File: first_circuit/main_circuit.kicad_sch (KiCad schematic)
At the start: 3 parts

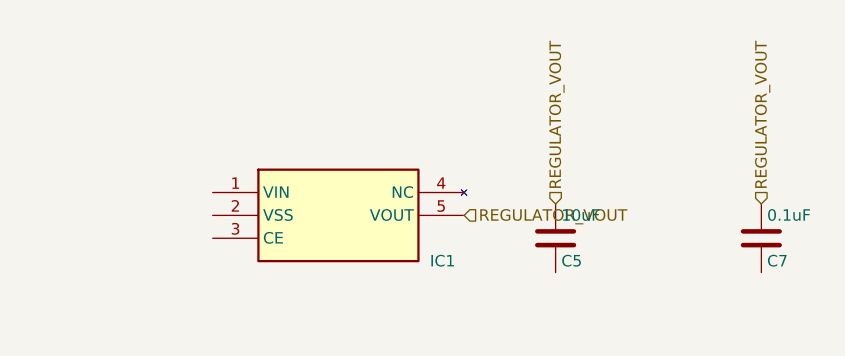
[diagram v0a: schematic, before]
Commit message: start again
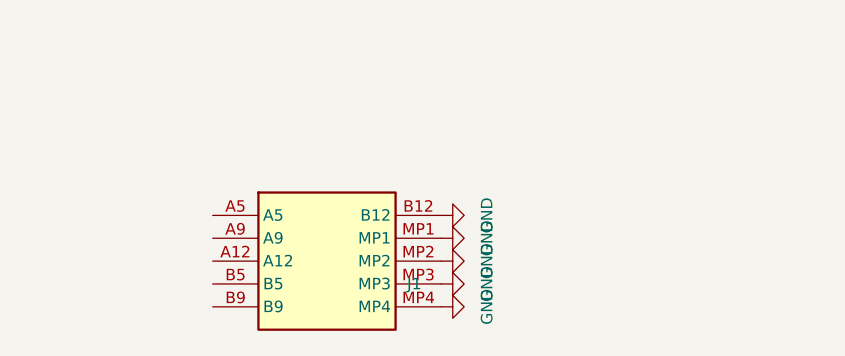
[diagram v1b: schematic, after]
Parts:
- removed C5: 10uF, Capacitor_SMD:C_0201_0603Metric, symbol Device:C
- removed C7: 0.1uF, Capacitor_SMD:C_0201_0603Metric, symbol Device:C
- removed IC1: (no value), SamacSys_Parts:SOT95P280X130-5N, symbol SamacSys_Parts:XC6220B331MR-G
- added J1: (no value), SamacSys_Parts:USB4135GFA, symbol SamacSys_Parts:USB4135-GF-A
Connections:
- new net GND: J1.B12, J1.MP1, J1.MP2, J1.MP3, J1.MP4

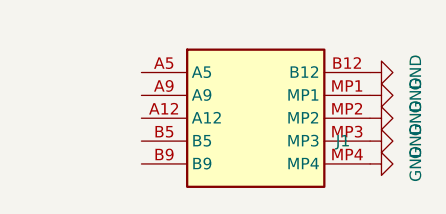
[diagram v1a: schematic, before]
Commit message: rc_delay
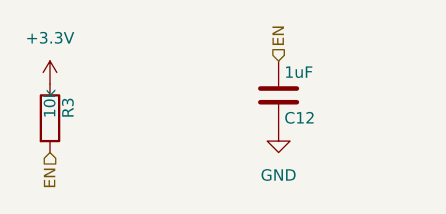
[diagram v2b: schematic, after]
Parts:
- removed J1: (no value), SamacSys_Parts:USB4135GFA, symbol SamacSys_Parts:USB4135-GF-A
- added C12: 1uF, Capacitor_SMD:C_0603_1608Metric, symbol Device:C
- added R3: 10k, Resistor_SMD:R_0603_1608Metric, symbol Device:R
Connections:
- net GND: now also C12.2
- new net +3.3V: R3.1
- new net EN: C12.1, R3.2
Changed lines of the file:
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@@
 	)
 	(symbol
-		(lib_id "SamacSys_Parts:USB4135-GF-A")
-		(at 40.64 30.48 0)
-		(unit 1)
-		(exclude_from_sim no)
-		(in_bom yes)
-		(on_board yes)
-		(dnp no)
-		(fields_autoplaced no)
-		(property "Reference" "J1"
-			(at 62.23 38.1 0.0000)
-			(effects
-				(font
-					(size 1.27 1.27)
-				)
-				(justify left)
-			)
-		)
-		(property "Footprint" "SamacSys_Parts:USB4135GFA"
-			(at 62.23 -64.44 0.0000)
-			(effects
-				(font
-					(size 1.27 1.27)
-				)
-				(hide yes)
-			)
-		)
-		(property "hierarchy_path" "/74824406-cd07-43be-b55f-f7d501532b0e"
-			(at 43.18 35.5599 0)
+		(lib_id "Device:R")
+		(at 30.48 35.56 0)
+		(unit 1)
+		(exclude_from_sim no)
+		(in_bom yes)
+		(on_board yes)
+		(dnp no)
+		(fields_autoplaced no)
+		(property "Reference" "R3"
+			(at 32.512 35.56 90)
+			(effects
+				(font
+					(size 1.27 1.27)
+				)
+				(justify left)
+			)
+		)
+		(property "Value" "10k"
+			(at 30.48 35.56 90)
+			(effects
+				(font
+					(size 1.27 1.27)
+				)
+				(justify left)
+			)
+		)
+		(property "Footprint" "Resistor_SMD:R_0603_1608Metric"
+			(at 28.702 35.56 90)
+			(effects
+				(font
+					(size 1.27 1.27)
+				)
+				(hide yes)
+			)
+		)
+		(property "hierarchy_path" "/18790e42-201e-4808-bfa1-f33409c8c696"
+			(at 33.02 40.6399 0)
 			(effects
 				(font
@@
 		)
 		(property "project_name" "main_circuit"
-			(at 43.18 35.5599 0)
-			(effects
-				(font
-					(size 1.27 1.27)
-				)
-				(hide yes)
-			)
-		)
-		(property "root_uuid" "74824406-cd07-43be-b55f-f7d501532b0e"
-			(at 43.18 35.5599 0)
-			(effects
-				(font
-					(size 1.27 1.27)
-				)
-				(hide yes)
-			)
-		)
-		(pin "A5"
-		)
-		(pin "A9"
-		)
-		(pin "A12"
-		)
-		(pin "B5"
-		)
-		(pin "B9"
-		)
-		(pin "B12"
-		)
-		(pin "MP1"
-		)
-		(pin "MP2"
-		)
-		(pin "MP3"
-		)
-		(pin "MP4"
-		)
-		(instances
-			(project ""
-				(path "/74824406-cd07-43be-b55f-f7d501532b0e"
-					(reference "J1")
-					(unit 1)
-				)
-			)
-		)
-	)
-	(symbol
-		(lib_id "power:GND")
-		(at 66.04 30.48 90)
+			(at 33.02 40.6399 0)
+			(effects
+				(font
+					(size 1.27 1.27)
+				)
+				(hide yes)
+			)
+		)
+		(property "root_uuid" "18790e42-201e-4808-bfa1-f33409c8c696"
+			(at 33.02 40.6399 0)
+			(effects
+				(font
+					(size 1.27 1.27)
+				)
+				(hide yes)
+			)
+		)
+		(pin "1"
+		)
+		(pin "2"
+		)
+		(instances
+			(project ""
+				(path "/18790e42-201e-4808-bfa1-f33409c8c696"
+					(reference "R3")
+					(unit 1)
+				)
+			)
+		)
+	)
+	(symbol
+		(lib_id "Device:C")
+		(at 55.88 33.02 0)
+		(unit 1)
+		(exclude_from_sim no)
+		(in_bom yes)
+		(on_board yes)
+		(dnp no)
+		(fields_autoplaced no)
+		(property "Reference" "C12"
+			(at 56.515 35.56 0.0000)
+			(effects
+				(font
+					(size 1.27 1.27)
+				)
+				(justify left)
+			)
+		)
+		(property "Value" "1uF"
+			(at 56.515 30.48 0.0000)
+			(effects
+				(font
+					(size 1.27 1.27)
+				)
+				(justify left)
+			)
+		)
+		(property "Footprint" "Capacitor_SMD:C_0603_1608Metric"
+			(at 56.8452 29.21 0.0000)
+			(effects
+				(font
+					(size 1.27 1.27)
+				)
+				(hide yes)
+			)
+		)
+		(property "hierarchy_path" "/18790e42-201e-4808-bfa1-f33409c8c696"
+			(at 58.42 38.0999 0)
+			(effects
+				(font
+					(size 1.27 1.27)
+				)
+				(hide yes)
+			)
+		)
+		(property "project_name" "main_circuit"
+			(at 58.42 38.0999 0)
+			(effects
+				(font
+					(size 1.27 1.27)
+				)
+				(hide yes)
+			)
+		)
+		(property "root_uuid" "18790e42-201e-4808-bfa1-f33409c8c696"
+			(at 58.42 38.0999 0)
+			(effects
+				(font
+					(size 1.27 1.27)
+				)
+				(hide yes)
+			)
+		)
+		(pin "1"
+		)
+		(pin "2"
+		)
+		(instances
+			(project ""
+				(path "/18790e42-201e-4808-bfa1-f33409c8c696"
+					(reference "C12")
+					(unit 1)
+				)
+			)
+		)
+	)
+	(symbol
+		(lib_id "power:+3V3")
+		(at 30.48 31.75 0)
 		(unit 1)
 		(exclude_from_sim no)
@@
 		(fields_autoplaced no)
 		(property "Reference" "#PWR001"
-			(at 72.39 30.48 90)
-			(effects
-				(font
-					(size 1.27 1.27)
-				)
-				(justify left)
-				(hide yes)
-			)
-		)
-		(property "Value" "GND"
-			(at 71.11999999999999 30.48 0)
+			(at 30.48 27.94 0.0000)
+			(effects
+				(font
+					(size 1.27 1.27)
+				)
+				(justify left)
+				(hide yes)
+			)
+		)
+		(property "Value" "+3.3V"
+			(at 30.48 26.67 0)
 			(effects
 				(font
@@
 		)
 		(property "Footprint" ""
-			(at 66.04 30.48 0.0000)
+			(at 30.48 31.75 0.0000)
 			(effects
 				(font
@@
 	(symbol
 		(lib_id "power:GND")
-		(at 66.04 33.02 90)
+		(at 55.88 36.83 0)
 		(unit 1)
 		(exclude_from_sim no)
@@
 		(fields_autoplaced no)
 		(property "Reference" "#PWR002"
-			(at 72.39 33.02 90)
+			(at 55.88 30.48 0.0000)
 			(effects
 				(font
@@
 		)
 		(property "Value" "GND"
-			(at 71.11999999999999 33.02 0)
+			(at 55.88 41.910000000000004 0)
 			(effects
 				(font
@@
 		)
 		(property "Footprint" ""
-			(at 66.04 33.02 0.0000)
+			(at 55.88 36.83 0.0000)
 			(effects
 				(font
@@
 		)
 	)
-	(symbol
-		(lib_id "power:GND")
-		(at 66.04 35.56 90)
-		(unit 1)
-		(exclude_from_sim no)
-		(in_bom yes)
-		(on_board yes)
-		(dnp no)
-		(fields_autoplaced no)
-		(property "Reference" "#PWR003"
-			(at 72.39 35.56 90)
-			(effects
-				(font
-					(size 1.27 1.27)
-				)
-				(justify left)
-				(hide yes)
-			)
-		)
-		(property "Value" "GND"
-			(at 71.11999999999999 35.56 0)
-			(effects
-				(font
-					(size 1.27 1.27)
-				)
-			)
-		)
-		(property "Footprint" ""
-			(at 66.04 35.56 0.0000)
-			(effects
-				(font
-					(size 1.27 1.27)
-				)
-				(hide yes)
-			)
-		)
-		(pin "1"
-		)
-		(instances
-			(project ""
-				(path "/"
-					(reference "#PWR003")
-					(unit 1)
-				)
-			)
-		)
-	)
-	(symbol
-		(lib_id "power:GND")
-		(at 66.04 38.1 90)
-		(unit 1)
-		(exclude_from_sim no)
-		(in_bom yes)
-		(on_board yes)
-		(dnp no)
-		(fields_autoplaced no)
-		(property "Reference" "#PWR004"
-			(at 72.39 38.1 90)
-			(effects
-				(font
-					(size 1.27 1.27)
-				)
-				(justify left)
-				(hide yes)
-			)
-		)
-		(property "Value" "GND"
-			(at 71.11999999999999 38.1 0)
-			(effects
-				(font
-					(size 1.27 1.27)
-				)
-			)
-		)
-		(property "Footprint" ""
-			(at 66.04 38.1 0.0000)
-			(effects
-				(font
-					(size 1.27 1.27)
-				)
-				(hide yes)
-			)
-		)
-		(pin "1"
-		)
-		(instances
-			(project ""
-				(path "/"
-					(reference "#PWR004")
-					(unit 1)
-				)
-			)
-		)
-	)
-	(symbol
-		(lib_id "power:GND")
-		(at 66.04 40.64 90)
-		(unit 1)
-		(exclude_from_sim no)
-		(in_bom yes)
-		(on_board yes)
-		(dnp no)
-		(fields_autoplaced no)
-		(property "Reference" "#PWR005"
-			(at 72.39 40.64 90)
-			(effects
-				(font
-					(size 1.27 1.27)
-				)
-				(justify left)
-				(hide yes)
-			)
-		)
-		(property "Value" "GND"
-			(at 71.11999999999999 40.64 0)
-			(effects
-				(font
-					(size 1.27 1.27)
-				)
-			)
-		)
-		(property "Footprint" ""
-			(at 66.04 40.64 0.0000)
-			(effects
-				(font
-					(size 1.27 1.27)
-				)
-				(hide yes)
-			)
-		)
-		(pin "1"
-		)
-		(instances
-			(project ""
-				(path "/"
-					(reference "#PWR005")
-					(unit 1)
-				)
-			)
-		)
-	)
+	(hierarchical_label "EN"
+		(shape input)
+		(at 30.48 39.37 270)
+		(effects
+			(font
+				(size 1.27 1.27)
+			)
+			(justify right)
+		)
+	)
+	(hierarchical_label "EN"
+		(shape input)
+		(at 55.88 29.21 90)
+		(effects
+			(font
+				(size 1.27 1.27)
+			)
+			(justify left)
+		)
+	)

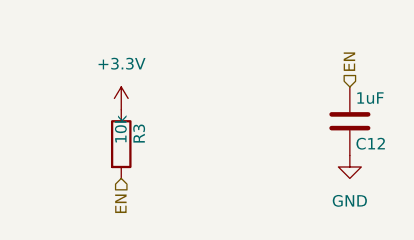
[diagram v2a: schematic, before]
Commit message: uart
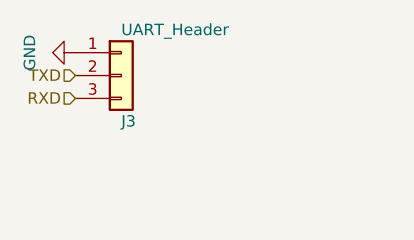
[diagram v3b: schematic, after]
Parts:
- removed C12: 1uF, Capacitor_SMD:C_0603_1608Metric, symbol Device:C
- removed R3: 10k, Resistor_SMD:R_0603_1608Metric, symbol Device:R
- added J3: UART_Header, Connector_PinHeader_2.54mm:PinHeader_1x03_P2.54mm_Vertical, symbol Connector_Generic:Conn_01x03
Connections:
- net GND: now also J3.1 (Pin_1)
- new net RXD: J3.3 (Pin_3)
- new net TXD: J3.2 (Pin_2)
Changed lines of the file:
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@@
 	)
 	(symbol
-		(lib_id "Device:R")
-		(at 30.48 35.56 0)
+		(lib_id "Connector_Generic:Conn_01x03")
+		(at 30.48 27.94 0)
 		(unit 1)
 		(exclude_from_sim no)
@@
 		(dnp no)
 		(fields_autoplaced no)
-		(property "Reference" "R3"
-			(at 32.512 35.56 90)
+		(property "Reference" "J3"
+			(at 30.48 33.02 0.0000)
 			(effects
 				(font
@@
 			)
 		)
-		(property "Value" "10k"
-			(at 30.48 35.56 90)
+		(property "Value" "UART_Header"
+			(at 30.48 22.86 0.0000)
 			(effects
 				(font
@@
 			)
 		)
-		(property "Footprint" "Resistor_SMD:R_0603_1608Metric"
-			(at 28.702 35.56 90)
+		(property "Footprint" "Connector_PinHeader_2.54mm:PinHeader_1x03_P2.54mm_Vertical"
+			(at 30.48 27.94 0.0000)
 			(effects
 				(font
@@
 			)
 		)
-		(property "hierarchy_path" "/18790e42-201e-4808-bfa1-f33409c8c696"
-			(at 33.02 40.6399 0)
+		(property "hierarchy_path" "/d6d32006-2e24-439e-8123-b988d5d2a167"
+			(at 33.02 33.0199 0)
 			(effects
 				(font
@@
 		)
 		(property "project_name" "main_circuit"
-			(at 33.02 40.6399 0)
+			(at 33.02 33.0199 0)
 			(effects
 				(font
@@
 			)
 		)
-		(property "root_uuid" "18790e42-201e-4808-bfa1-f33409c8c696"
-			(at 33.02 40.6399 0)
+		(property "root_uuid" "d6d32006-2e24-439e-8123-b988d5d2a167"
+			(at 33.02 33.0199 0)
 			(effects
 				(font
@@
 		(pin "2"
 		)
+		(pin "3"
+		)
 		(instances
 			(project ""
-				(path "/18790e42-201e-4808-bfa1-f33409c8c696"
-					(reference "R3")
+				(path "/d6d32006-2e24-439e-8123-b988d5d2a167"
+					(reference "J3")
 					(unit 1)
 				)
@@
 	)
 	(symbol
-		(lib_id "Device:C")
-		(at 55.88 33.02 0)
-		(unit 1)
-		(exclude_from_sim no)
-		(in_bom yes)
-		(on_board yes)
-		(dnp no)
-		(fields_autoplaced no)
-		(property "Reference" "C12"
-			(at 56.515 35.56 0.0000)
-			(effects
-				(font
-					(size 1.27 1.27)
-				)
-				(justify left)
-			)
-		)
-		(property "Value" "1uF"
-			(at 56.515 30.48 0.0000)
-			(effects
-				(font
-					(size 1.27 1.27)
-				)
-				(justify left)
-			)
-		)
-		(property "Footprint" "Capacitor_SMD:C_0603_1608Metric"
-			(at 56.8452 29.21 0.0000)
-			(effects
-				(font
-					(size 1.27 1.27)
-				)
-				(hide yes)
-			)
-		)
-		(property "hierarchy_path" "/18790e42-201e-4808-bfa1-f33409c8c696"
-			(at 58.42 38.0999 0)
-			(effects
-				(font
-					(size 1.27 1.27)
-				)
-				(hide yes)
-			)
-		)
-		(property "project_name" "main_circuit"
-			(at 58.42 38.0999 0)
-			(effects
-				(font
-					(size 1.27 1.27)
-				)
-				(hide yes)
-			)
-		)
-		(property "root_uuid" "18790e42-201e-4808-bfa1-f33409c8c696"
-			(at 58.42 38.0999 0)
-			(effects
-				(font
-					(size 1.27 1.27)
-				)
-				(hide yes)
-			)
-		)
-		(pin "1"
-		)
-		(pin "2"
-		)
-		(instances
-			(project ""
-				(path "/18790e42-201e-4808-bfa1-f33409c8c696"
-					(reference "C12")
-					(unit 1)
-				)
-			)
-		)
-	)
-	(symbol
-		(lib_id "power:+3V3")
-		(at 30.48 31.75 0)
+		(lib_id "power:GND")
+		(at 25.4 25.4 270)
 		(unit 1)
 		(exclude_from_sim no)
@@
 		(fields_autoplaced no)
 		(property "Reference" "#PWR001"
-			(at 30.48 27.94 0.0000)
+			(at 19.05 25.4 270)
 			(effects
 				(font
@@
 			)
 		)
-		(property "Value" "+3.3V"
-			(at 30.48 26.67 0)
+		(property "Value" "GND"
+			(at 20.32 25.400000000000002 0)
 			(effects
 				(font
@@
 		)
 		(property "Footprint" ""
-			(at 30.48 31.75 0.0000)
+			(at 25.4 25.4 0.0000)
 			(effects
 				(font
@@
 		)
 	)
-	(symbol
-		(lib_id "power:GND")
-		(at 55.88 36.83 0)
-		(unit 1)
-		(exclude_from_sim no)
-		(in_bom yes)
-		(on_board yes)
-		(dnp no)
-		(fields_autoplaced no)
-		(property "Reference" "#PWR002"
-			(at 55.88 30.48 0.0000)
-			(effects
-				(font
-					(size 1.27 1.27)
-				)
-				(justify left)
-				(hide yes)
-			)
-		)
-		(property "Value" "GND"
-			(at 55.88 41.910000000000004 0)
-			(effects
-				(font
-					(size 1.27 1.27)
-				)
-			)
-		)
-		(property "Footprint" ""
-			(at 55.88 36.83 0.0000)
-			(effects
-				(font
-					(size 1.27 1.27)
-				)
-				(hide yes)
-			)
-		)
-		(pin "1"
-		)
-		(instances
-			(project ""
-				(path "/"
-					(reference "#PWR002")
-					(unit 1)
-				)
-			)
-		)
-	)
-	(hierarchical_label "EN"
+	(hierarchical_label "TXD"
 		(shape input)
-		(at 30.48 39.37 270)
+		(at 25.4 27.94 180)
 		(effects
 			(font
@@
 		)
 	)
-	(hierarchical_label "EN"
+	(hierarchical_label "RXD"
 		(shape input)
-		(at 55.88 29.21 90)
+		(at 25.4 30.48 180)
 		(effects
 			(font
 				(size 1.27 1.27)
 			)
-			(justify left)
+			(justify right)
 		)
 	)
